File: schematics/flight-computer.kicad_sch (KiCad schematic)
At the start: 45 parts, among them J1 BATT, J2 SERIAL, J3 BLACKBOX, P1 SWD_TC, P2 GPS, P3 TLM, U1 MAX604, U10 MAX14787E, U11 MAX14787E, U12 NC7SZ04, U2 MAX604, U3 STM32F405RGT6, U9 CDCLVC1103PW, Y1 LFTCXO068373

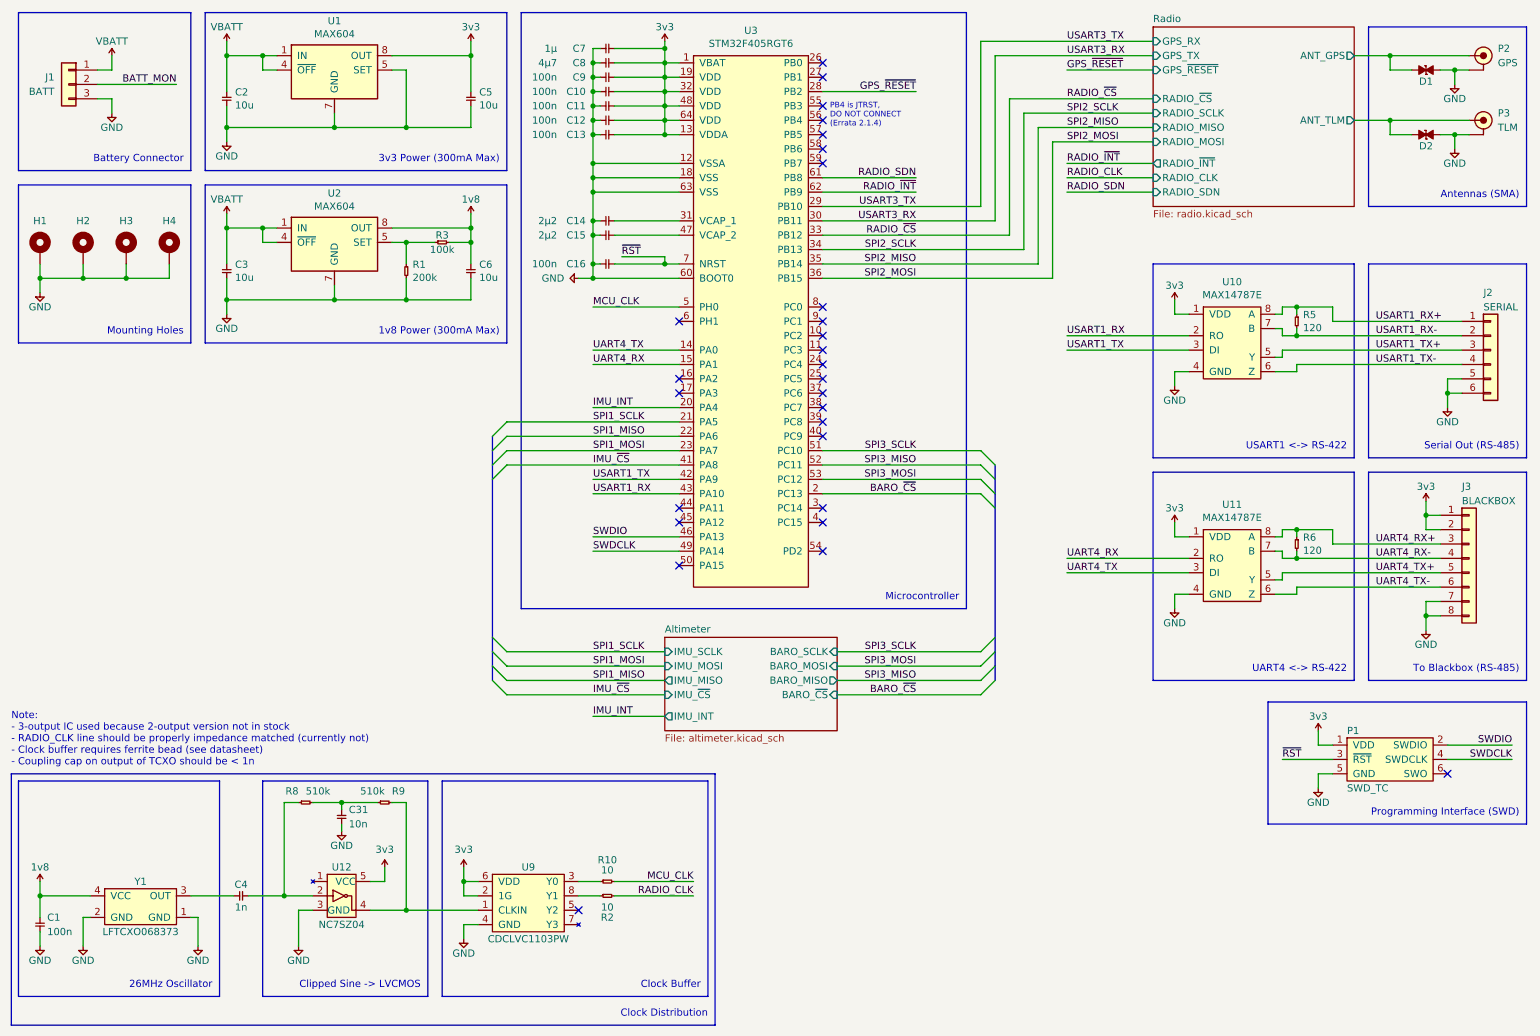
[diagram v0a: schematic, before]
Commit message: Complete revision 1 schematic
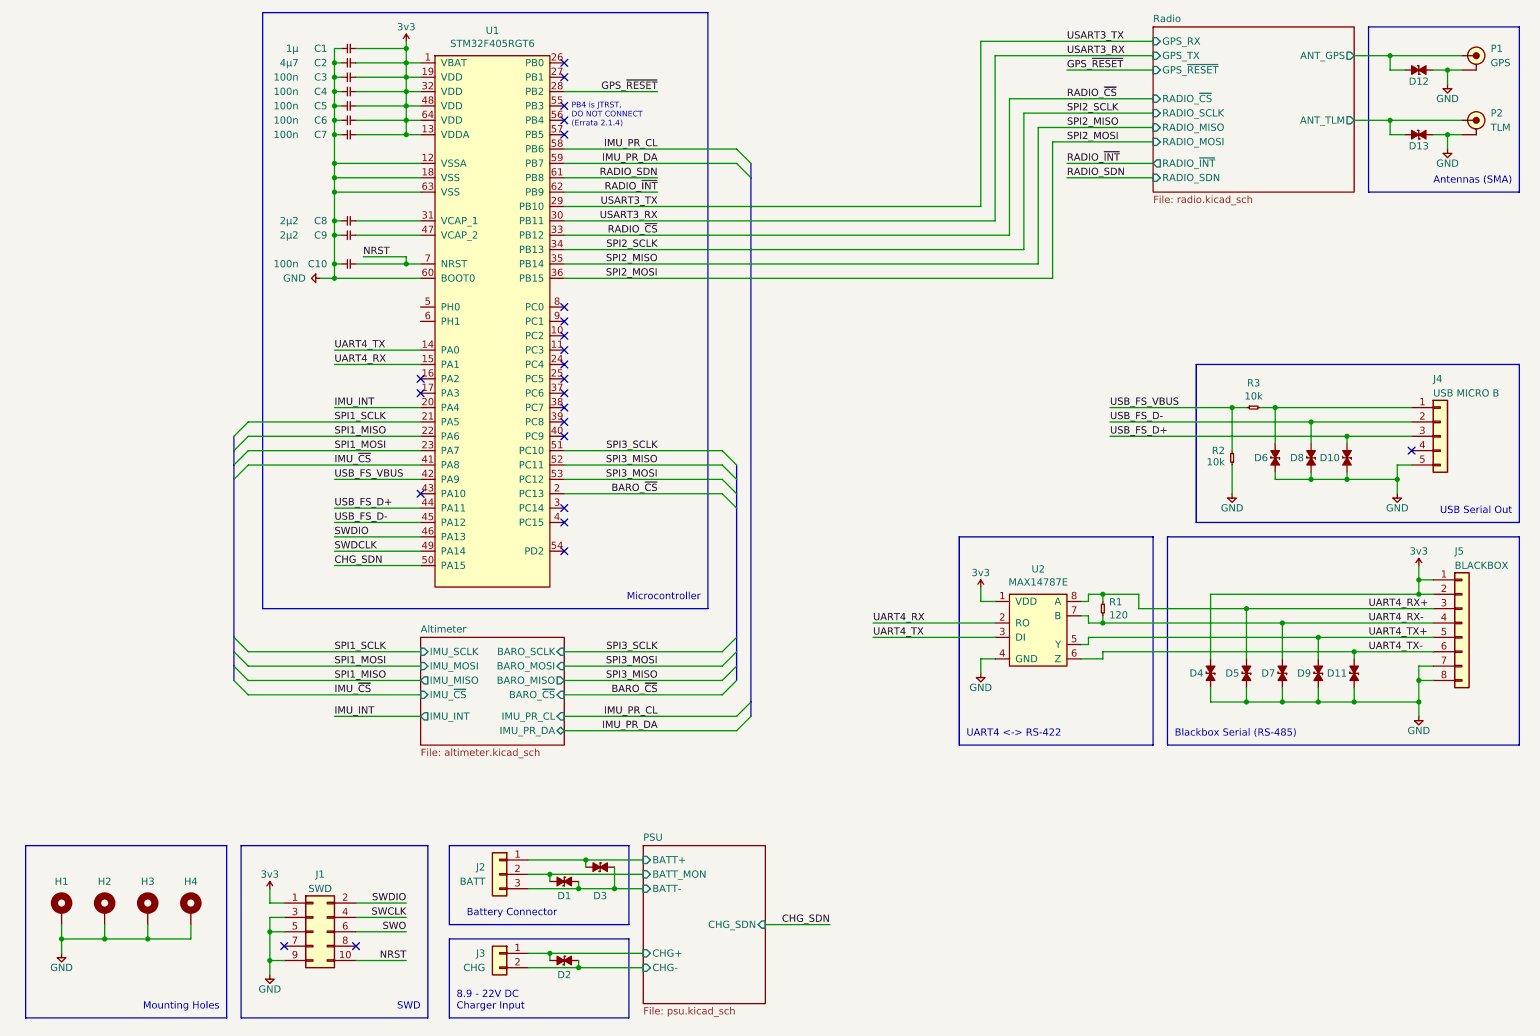
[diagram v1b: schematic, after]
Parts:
- removed C1: 100n, Strix:C_0402, symbol Strix:C
- removed C2, C3, C5, C6: 10u, Strix:C_0402, symbol Strix:C
- removed C31: 10n, Strix:C_0402, symbol Strix:C
- removed C4: 1n, Strix:C_0402, symbol Strix:C
- removed J2: SERIAL, Strix:Molex_Nano-Fit_105314-1106, symbol Strix:Conn_01x06
- removed P1: SWD_TC, Strix:SWD_TC, symbol Strix:SWD_TC
- removed R1: 200k, Strix:R_0402, symbol Strix:R
- removed R10: 10, Strix:R_0402, symbol Strix:R
- removed R5: 120, Strix:R_0402, symbol Strix:R
- removed R8, R9: 510k, Strix:R_0402, symbol Strix:R
- removed U1, U2: MAX604, Strix:MAX604, symbol Strix:MAX604
- removed U10: MAX14787E, Strix:MAX14787E, symbol Strix:MAX14787E
- removed U12: NC7SZ04, cusf:SOT-23-5, symbol Strix:NC7SZ04
- removed U9: CDCLVC1103PW, Strix:CDCLVC1103PW, symbol Strix:CDCLVC1103PW
- removed Y1: LFTCXO068373, Strix:LFTCXO068373, symbol Strix:LFTCXO068373
- added D1, D10, D11, D2, D3, D4, D5, D6, D7, D8, D9: ESD_DIODE, cusf:D_0402, symbol Strix:ESD_DIODE
- added J1: SWD, symbol Strix:Conn_02x05
- added J3: CHG, symbol Strix:Conn_01x02
- added J4: USB MICRO B, symbol Strix:Conn_01x05
- R2: value 10 -> 10k; footprint Strix:R_0402 -> (none)
- R3: value 100k -> 10k; footprint Strix:R_0402 -> (none)
- renumbered C7 to C1, C16 to C10, C8 to C2, C9 to C3, C10 to C4, C11 to C5, C12 to C6, C13 to C7, C14 to C8, C15 to C9, D1 to D12, D2 to D13, J1 to J2, J3 to J5, P2 to P1, P3 to P2, R6 to R1, U3 to U1, U11 to U2
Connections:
- net RADIO_CLK is gone; now on net USB_FS_VBUS: R2.2
- net USART1_TX is gone; now on net USB_FS_VBUS: U1.42 (PA9)
- net 3v3: now also D4.2, J1.1 (Pin_1)
- net GND: now also R2.1, D10.1, D11.1, D4.1, D5.1, D6.1, D7.1, D8.1, D9.1, J1.3 (Pin_3), J1.5 (Pin_5), J1.9 (Pin_9), J4.5 (Pin_5); no longer J2.3 (Pin_3)
- net SWDIO: now also J1.2 (Pin_2)
- net UART4_RX+: now also D5.2
- net UART4_RX-: now also D7.2
- net UART4_TX+: now also D9.2
- net UART4_TX-: now also D11.2
- net USB_FS_VBUS: now reaches R3.1
- net USB_FS_D+: now reaches U1.44 (PA11)
- net USB_FS_D+: now also D10.2, J4.3 (Pin_3)
- net USB_FS_D-: now reaches U1.45 (PA12)
- net USB_FS_D-: now also D8.2, J4.2 (Pin_2)
- net CHG_SDN: now reaches U1.50 (PA15)
- net IMU_PR_CL: now reaches U1.58 (PB6)
- net IMU_PR_DA: now reaches U1.59 (PB7)
- net 1v8: no longer names the net of R3.2
- net 1v8: now also D6.2, J4.1 (Pin_1)
- net BATT_MON renamed PSU/BATT_MON
- net PSU/BATT_MON: now also D1.1
- net MCU_CLK: no longer names the net of U1.5 (PH0)
- net USART1_RX: no longer names the net of U1.43 (PA10)
- net VBATT renamed PSU/BATT+
- net PSU/BATT+: now also D3.1
- net ~{RST} renamed NRST
- net NRST: now also J1.10 (Pin_10)
- new net PSU/BATT-: D1.2, D3.2, J2.3 (Pin_3)
- new net PSU/CHG+: D2.1, J3.1 (Pin_1)
- new net PSU/CHG-: D2.2, J3.2 (Pin_2)
- new net SWCLK: J1.4 (Pin_4)
- new net SWO: J1.6 (Pin_6)
- no-connect marks 28 -> 24
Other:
- added sheet PSU (psu.kicad_sch)
- sheet Altimeter ports: added IMU_PR_CL, IMU_PR_DA; removed none
- sheet Radio ports: added none; removed RADIO_CLK
- note added: "8.9 - 22V DC Charger Input"
- note added: "Blackbox Serial (RS-485)"
- note added: "SWD"
- note added: "USB Serial Out"
- note removed: "1v8 Power (300mA Max)"
- note removed: "26MHz Oscillator"
- note removed: "3v3 Power (300mA Max)"
- note removed: "Clipped Sine -> LVCMOS"
- note removed: "Clock Buffer"
- note removed: "Clock Distribution"
- note removed: "Note: - 3-output IC used because 2-output version not in stock - RADIO_CLK line should be properly impedance matched (currently not) - Clock buffer requires ferrite bead (see datasheet) - Coupling cap on output of TCXO should be < 1n"
- note removed: "Programming Interface (SWD)"
- note removed: "Serial Out (RS-485)"
- note removed: "To Blackbox (RS-485)"
- note removed: "USART1 <-> RS-422"
- moved on the sheet: C1, C10, C2, C3, C4, C5, C6, C7, C8, C9, D12, D13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
